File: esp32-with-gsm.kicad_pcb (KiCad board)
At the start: 2 copper layers, 101.6 x 61 mm, 32 parts, among them J1 LCD, J2 Bat Etx, J3 SPI Etx, J5 Power in, Q1 BC548, U1 ESP32-DEVKITC-32D, U2 SIM800L-CORE

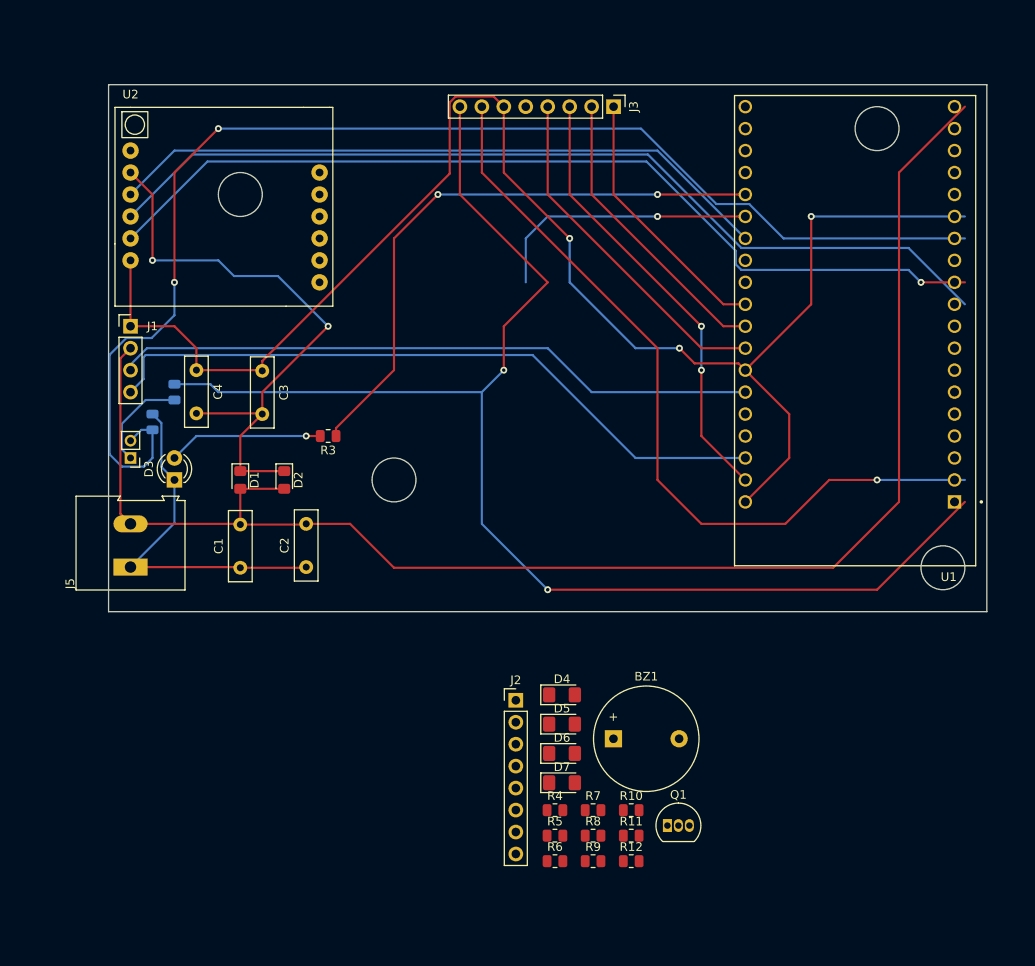
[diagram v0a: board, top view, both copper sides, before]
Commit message: Added v2r1
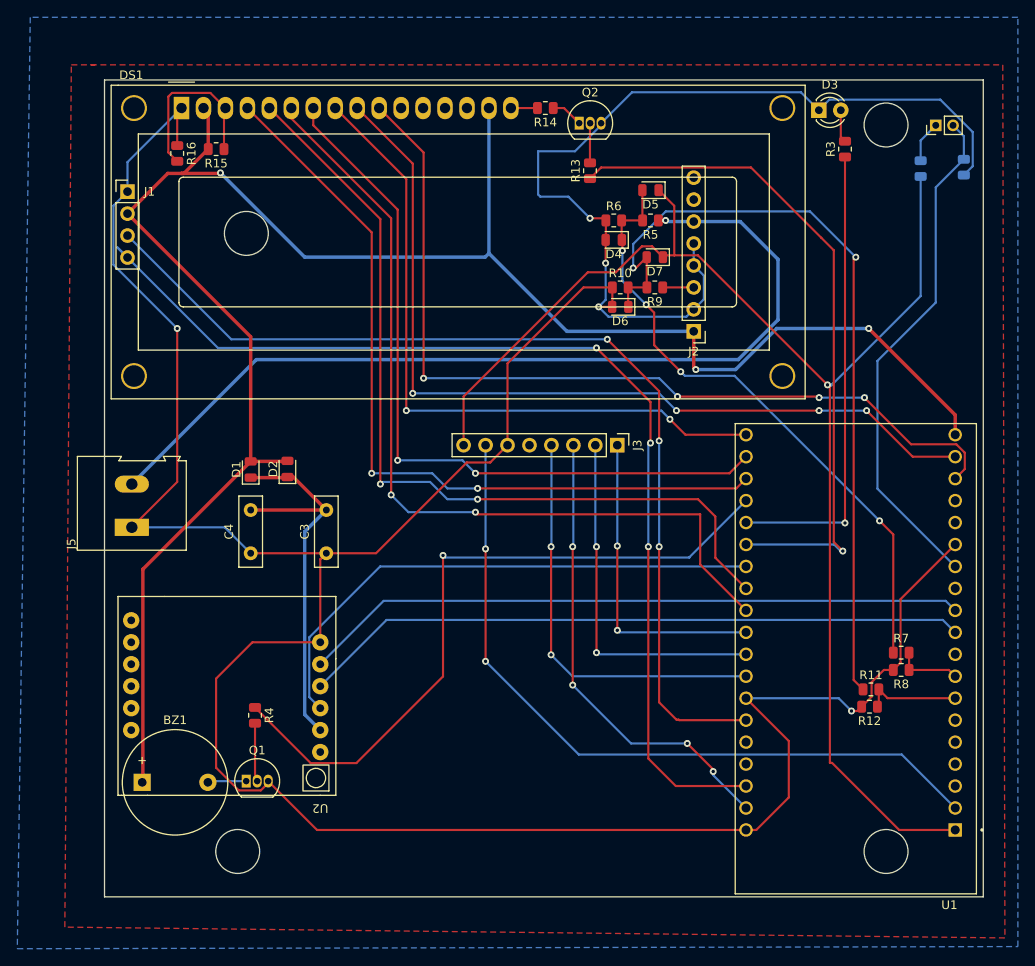
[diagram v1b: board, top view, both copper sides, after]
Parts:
- removed C1, C2: 1000uF, Capacitor_THT:C_Disc_D8.0mm_W2.5mm_P5.00mm
- added DS1: WC1602A, Display:WC1602A, F.Cu at (107.5, 53.5)
- added Q2: BC548, Package_TO_SOT_THT:TO-92_Inline, F.Cu at (153.5, 55.2)
- added R13: 1k, Resistor_SMD:R_0805_2012Metric, F.Cu at (154.8, 60.8)
- added R14: 1k, Resistor_SMD:R_0805_2012Metric, F.Cu at (149.6, 53.5)
- added R15: 1k, Resistor_SMD:R_0805_2012Metric, F.Cu at (111.5, 58.2)
- added R16: 1k, Resistor_SMD:R_0805_2012Metric, F.Cu at (107.0, 58.8)
- D1, D2: footprint Diode_SMD:D_0805_2012Metric_Pad1.15x1.40mm_HandSolder -> Diode_SMD:D_0805_2012Metric
- D4, D5, D6, D7: footprint Diode_SMD:D_1206_3216Metric_Pad1.42x1.75mm_HandSolder -> Diode_SMD:D_0805_2012Metric
- moved CFG1 100.8 mm to (194.8, 55.5), turned to 90 degrees
- moved R2 98.4 mm to (198.0, 60.3), turned to -90 degrees
- moved R1 90.1 mm to (193.0, 60.5), turned to 90 degrees
- moved D3 85.9 mm to (181.2, 53.8), turned to 0 degrees
- moved R6 74.4 mm to (157.5, 66.5)
- moved U2 73.0 mm to (123.5, 128.0), turned to 180 degrees
- moved R5 72.0 mm to (161.8, 66.5), turned to 180 degrees
- moved R3 68.4 mm to (184.2, 58.2), turned to 90 degrees
- moved R9 66.8 mm to (162.2, 74.2), turned to 180 degrees
- moved D5 62.6 mm to (161.8, 63.0), turned to 180 degrees
- moved D7 61.7 mm to (162.2, 70.8), turned to 180 degrees
- moved R10 60.5 mm to (158.2, 74.2)
- moved BZ1 54.7 mm to (103.0, 131.5)
- moved D4 53.0 mm to (157.5, 68.8), turned to 180 degrees
- moved D6 52.1 mm to (158.2, 76.5), turned to 180 degrees
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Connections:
- U1 pad J2-17: unconnected-(U1-SD3-PadJ2-17) -> LCD_DT4
- U1 pad J2-18: unconnected-(U1-CMD-PadJ2-18) -> LCD_DT3
- U1 pad J3-11: unconnected-(U1-IO17-PadJ3-11) -> LCD_EN
- U1 pad J3-12: unconnected-(U1-IO16-PadJ3-12) -> LCD_RW
- U1 pad J3-14: BUZZ -> LCD_BACKLIGHT
- U1 pad J3-16: unconnected-(U1-IO15-PadJ3-16) -> BUZZ
- U1 pad J3-17: unconnected-(U1-SD1-PadJ3-17) -> LCD_RS
- U1 pad J3-18: unconnected-(U1-SD0-PadJ3-18) -> LCD_DT1
- U1 pad J3-19: unconnected-(U1-CLK-PadJ3-19) -> LCD_DT2
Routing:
- net GND: track 221.0 -> 405.0 mm, vias 3 -> 5
- net Vin: track 0.00 -> 105.3 mm, vias 0 -> 1
- net LCD_DT4: track 0.00 -> 103.5 mm, vias 0 -> 4
- net LCD_DT3: track 0.00 -> 101.7 mm, vias 0 -> 4
- net LCD_EN: track 0.00 -> 99.5 mm, vias 0 -> 2
- net LCD_RW: track 0.00 -> 99.1 mm, vias 0 -> 2
- net Net-(D6-K): track 0.00 -> 92.9 mm, vias 0 -> 2
- net LCD_RS: track 0.00 -> 92.7 mm, vias 0 -> 2
- net CFG-BTN: track 148.5 -> 59.4 mm, vias 2 -> 0
- net LCD_DT1: track 0.00 -> 87.1 mm, vias 0 -> 2
- net LCD_BACKLIGHT: track 0.00 -> 79.4 mm, vias 0 -> 1
- net LCD_DT2: track 0.00 -> 78.9 mm, vias 0 -> 2
- net Net-(D4-K): track 0.00 -> 72.3 mm, vias 0 -> 4
- net +5V: track 173.6 -> 225.5 mm, vias 0 -> 3
- net BUZZ: track 31.5 -> 80.5 mm
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- added copper zone on B.Cu, net GND
- added copper zone on F.Cu, net GND
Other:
- board size 101.6 x 61 mm -> 101.7 x 94.5 mm
